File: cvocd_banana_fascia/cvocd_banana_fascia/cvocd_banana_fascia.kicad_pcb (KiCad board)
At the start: 2 copper layers, 230 x 95 mm, 1 part

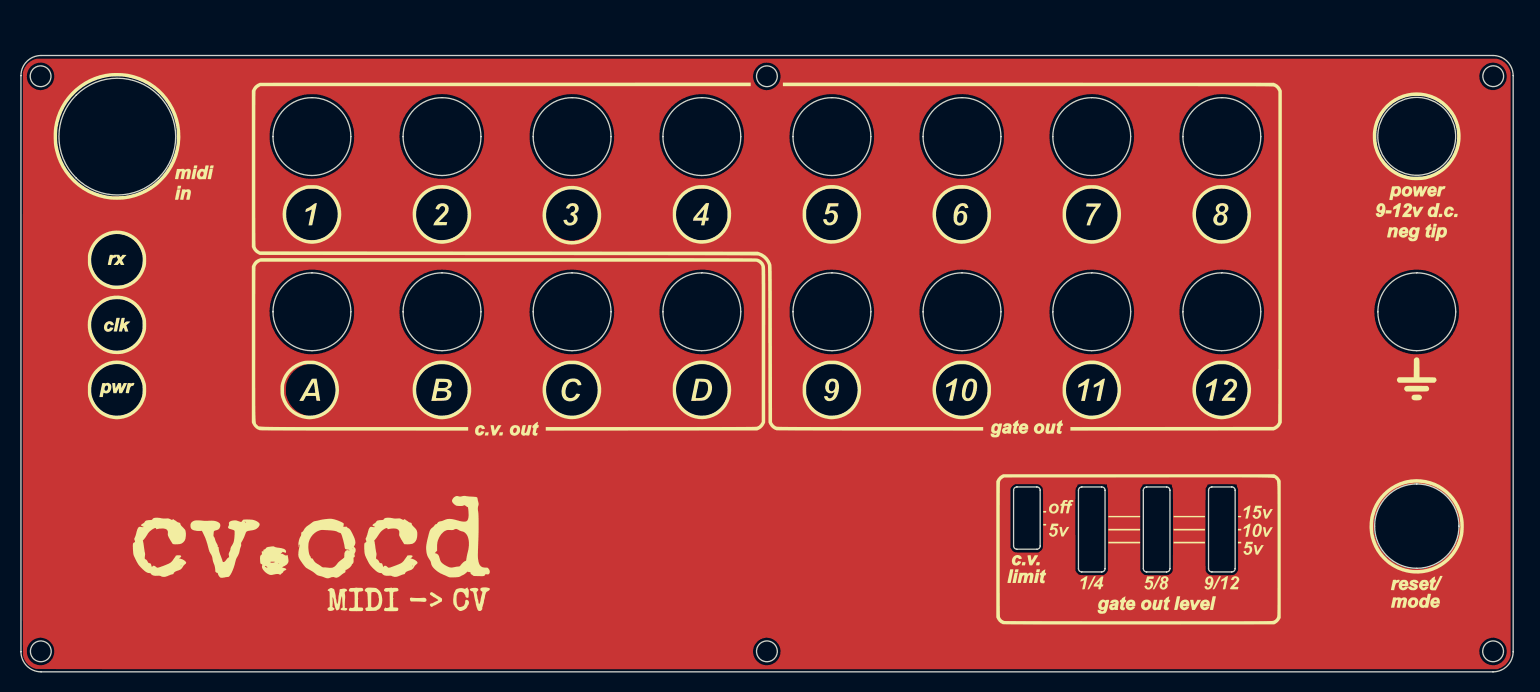
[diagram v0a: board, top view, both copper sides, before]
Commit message: banana pcb main v2
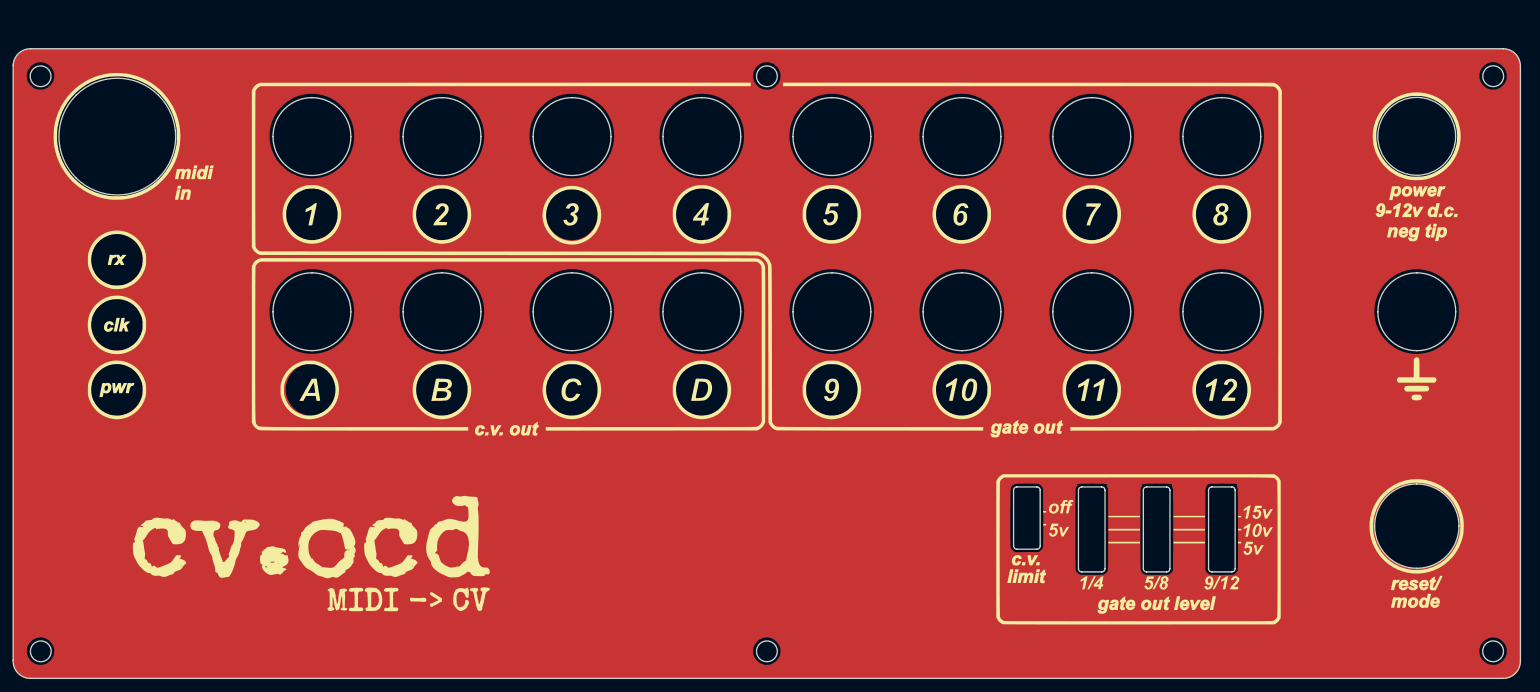
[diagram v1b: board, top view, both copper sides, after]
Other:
- board size 230 x 95 mm -> 232.3 x 97.1 mm

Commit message: PCB V2
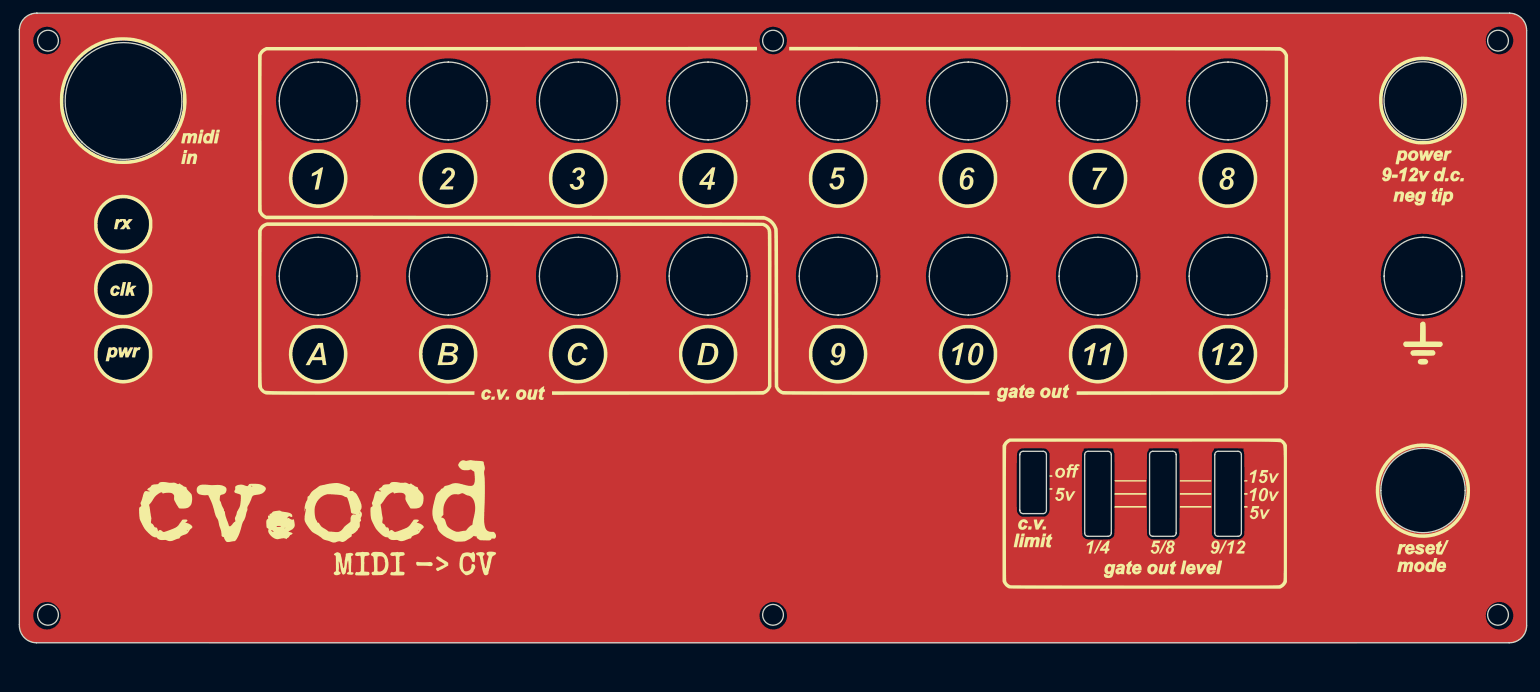
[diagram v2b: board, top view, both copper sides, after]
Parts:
- added REF**: MountingHole_3.2mm_M3, MountingHole:MountingHole_3.2mm_M3, F.Cu at (33.2, 141.8)
- added REF**: MountingHole_3.2mm_M3, MountingHole:MountingHole_3.2mm_M3, F.Cu at (256.8, 53.2)
- added REF**: MountingHole_3.2mm_M3, MountingHole:MountingHole_3.2mm_M3, F.Cu at (145.0, 141.8)
- added REF**: MountingHole_3.2mm_M3, MountingHole:MountingHole_3.2mm_M3, F.Cu at (33.2, 53.2)
- added REF**: MountingHole_3.2mm_M3, MountingHole:MountingHole_3.2mm_M3, F.Cu at (256.8, 141.8)
- added REF**: MountingHole_3.2mm_M3, MountingHole:MountingHole_3.2mm_M3, F.Cu at (145.0, 53.2)
- moved REF** 6.55 mm to (28.9, 146.0)
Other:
- outline, holes or cut-outs redrawn
